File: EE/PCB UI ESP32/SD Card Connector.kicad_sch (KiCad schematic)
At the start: 3 parts, among them U11 10067847001RLF

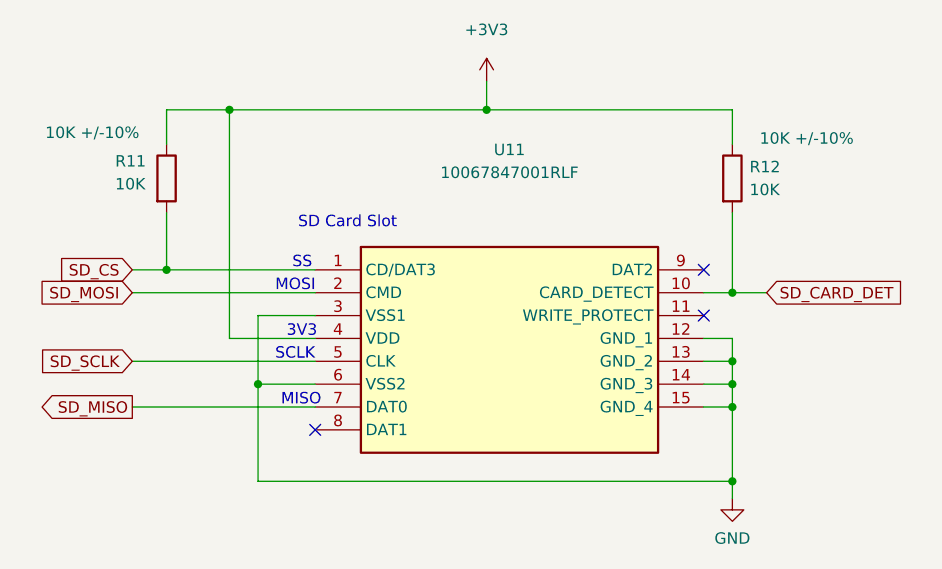
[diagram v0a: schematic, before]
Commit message: Finished V1 of ESP-UI
This is the version of ESP-UI that was ordered July 20 2025.
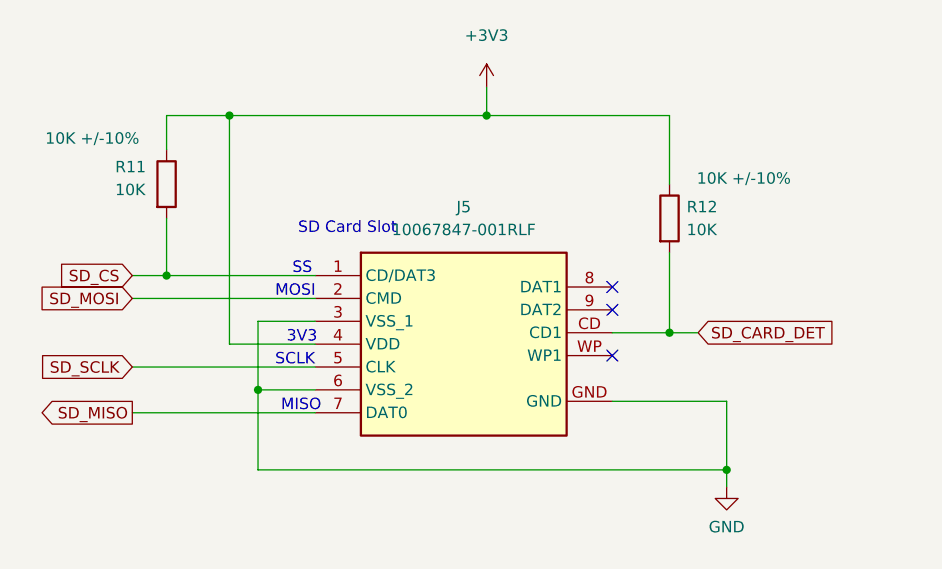
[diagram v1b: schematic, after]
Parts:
- removed U11: 10067847001RLF, DaisyBio_Mira:10067847001RLF, symbol 693063020911:693063020911
- added J5: 10067847-001RLF, DaisyBio_Mira:10067847001RLF, symbol DaisyBio_Mira:10067847-001RLF
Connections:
- net +3V3: now also J5.4 (VDD)
- net GND: now also J5.3 (VSS_1), J5.6 (VSS_2), J5.GND
- net SD_CARD_DET: now also J5.CD (CD1)
- net SD_CS: now also J5.1 (CD/DAT3)
- net SD_MISO: now also J5.7 (DAT0)
- net SD_MOSI: now also J5.2 (CMD)
- net SD_SCLK: now also J5.5 (CLK)
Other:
- moved on the sheet: R11, R12
